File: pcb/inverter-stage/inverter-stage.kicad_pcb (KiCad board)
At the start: 2 copper layers, 22 parts, among them J1 Screw_Terminal_01x02, J2 Conn_01x02, Q1 Q_NMOS_DGS, Q2 Q_NMOS_DGS, Q3 Q_NMOS_DGS, Q4 Q_NMOS_DGS, U1 IR2104, U2 IR2104, U3 L7805

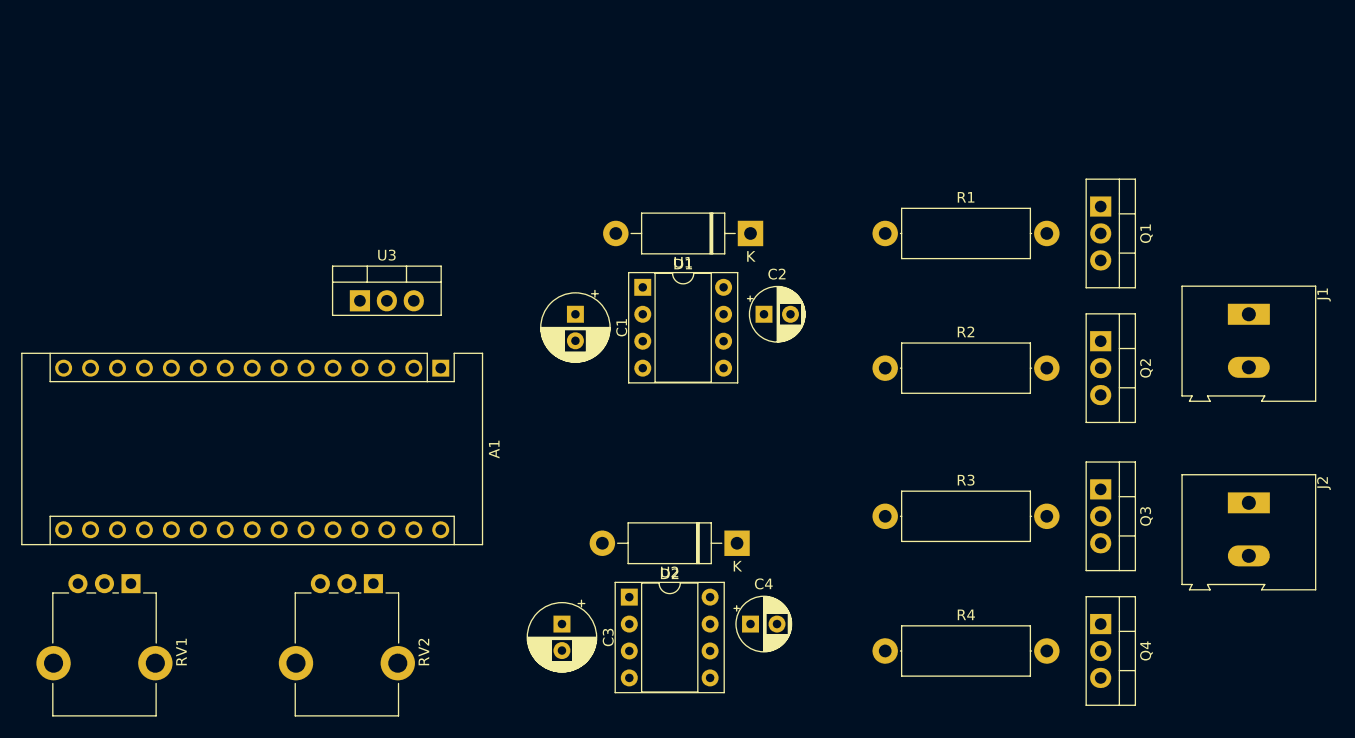
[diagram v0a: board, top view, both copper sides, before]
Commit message: start tracing
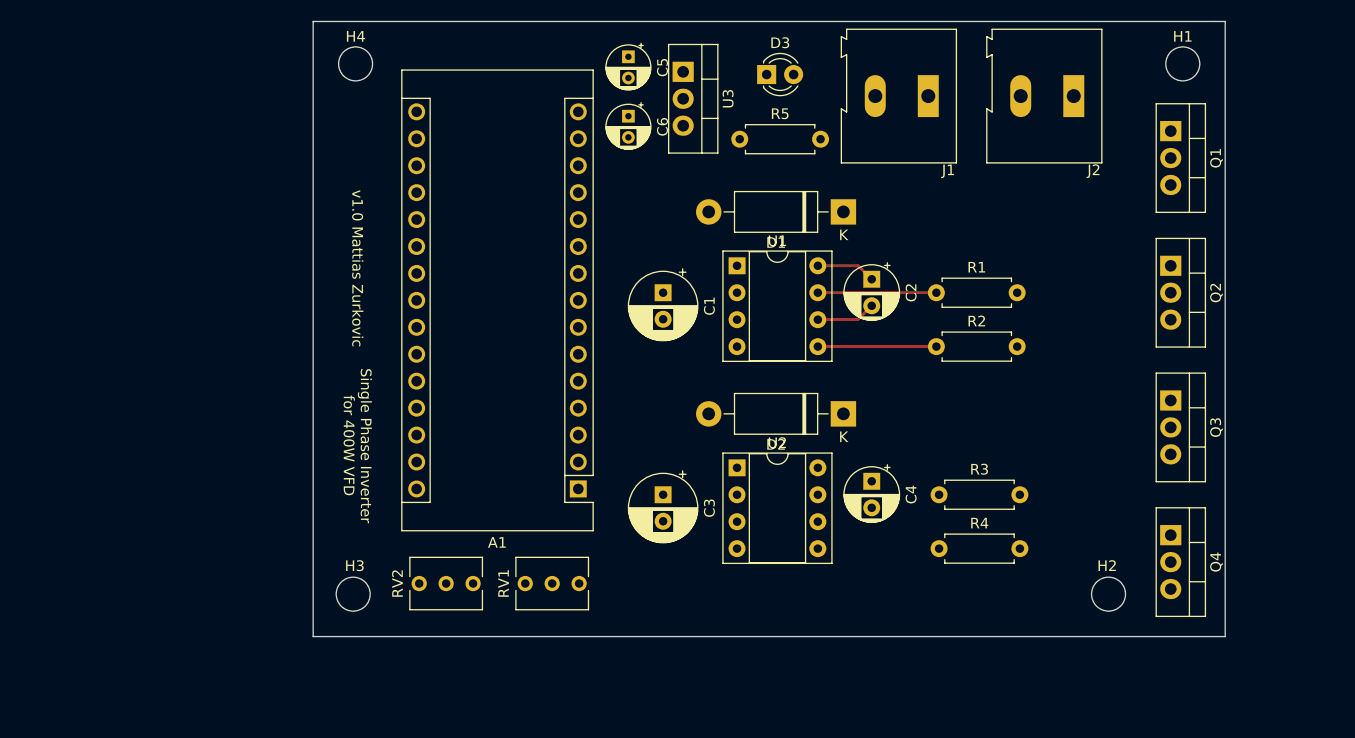
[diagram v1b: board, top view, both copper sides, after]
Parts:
- added C5: C, Capacitor_THT:CP_Radial_D4.0mm_P2.00mm, F.Cu at (130.7, 30.3)
- added C6: C, Capacitor_THT:CP_Radial_D4.0mm_P2.00mm, F.Cu at (130.7, 35.9)
- added D3: LED, LED_THT:LED_D3.0mm, F.Cu at (143.8, 32.0)
- added H1: MountingHole, MountingHole:MountingHole_3.2mm_M3, F.Cu at (183.0, 31.0)
- added H2: MountingHole, MountingHole:MountingHole_3.2mm_M3, F.Cu at (176.0, 81.0)
- added H3: MountingHole, MountingHole:MountingHole_3.2mm_M3, F.Cu at (104.8, 81.0)
- added H4: MountingHole, MountingHole:MountingHole_3.2mm_M3, F.Cu at (105.0, 31.0)
- added R5: R, Resistor_THT:R_Axial_DIN0207_L6.3mm_D2.5mm_P7.62mm_Horizontal, F.Cu at (141.2, 38.1)
- R1, R2, R3, R4: value R -> 100R; footprint Resistor_THT:R_Axial_DIN0414_L11.9mm_D4.5mm_P15.24mm_Horizontal -> Resistor_THT:R_Axial_DIN0207_L6.3mm_D2.5mm_P7.62mm_Horizontal
- RV1, RV2: footprint Potentiometer_THT:Potentiometer_Alpha_RD901F-40-00D_Single_Vertical_CircularHoles -> Potentiometer_THT:Potentiometer_Vishay_T73XW_Horizontal
- moved J2 41.8 mm to (172.7, 34.0), turned to 180 degrees
- moved U3 37.4 mm to (135.9, 31.8), turned to 270 degrees
- moved RV1 37.2 mm to (121.0, 80.0), turned to 90 degrees
- moved J1 36.6 mm to (159.0, 34.0), turned to 180 degrees
- moved C4 17.7 mm to (153.7, 70.4), turned to 270 degrees
- moved A1 17.3 mm to (126.0, 71.1), turned to 180 degrees
- moved U2 15.9 mm to (141.0, 69.1)
- moved D2 15.8 mm to (151.0, 64.0)
- moved C3 15.5 mm to (134.0, 71.6)
- moved R4 10.9 mm to (160.0, 76.7)
- moved C2 10.7 mm to (153.7, 51.3), turned to 270 degrees
- moved Q3 10.7 mm to (181.9, 62.7)
- moved Q4 10.7 mm to (181.9, 75.4)
- moved Q1 9.71 mm to (181.9, 37.3)
- moved Q2 9.71 mm to (181.9, 50.0)
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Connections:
- RV1 pad 1: +5V -> Net-(A1-Pad27)
- RV2 pad 1: +5V -> Net-(A1-Pad27)
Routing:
- net LO_A: track 0.00 -> 11.2 mm
- net HO_A: track 0.00 -> 11.2 mm
- net A: track 0.00 -> 5.62 mm
- net Net-(C2-Pad1): track 0.00 -> 5.61 mm
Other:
- board outline added: 86 x 58 mm
- net class Power added: clearance 1, trace_width 7.62, via_dia 0.8, via_drill 0.4
- board text added: "Single Phase Inverter for 400W VFD"
- board text added: "v1.0 Mattias Zurkovic"
